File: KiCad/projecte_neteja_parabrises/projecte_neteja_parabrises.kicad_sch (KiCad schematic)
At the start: 0 parts

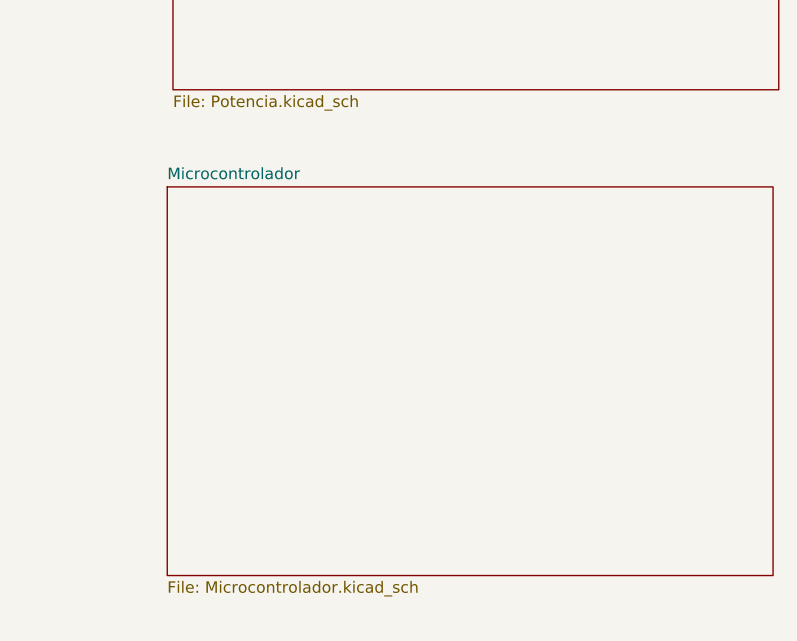
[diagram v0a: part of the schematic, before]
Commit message: huella
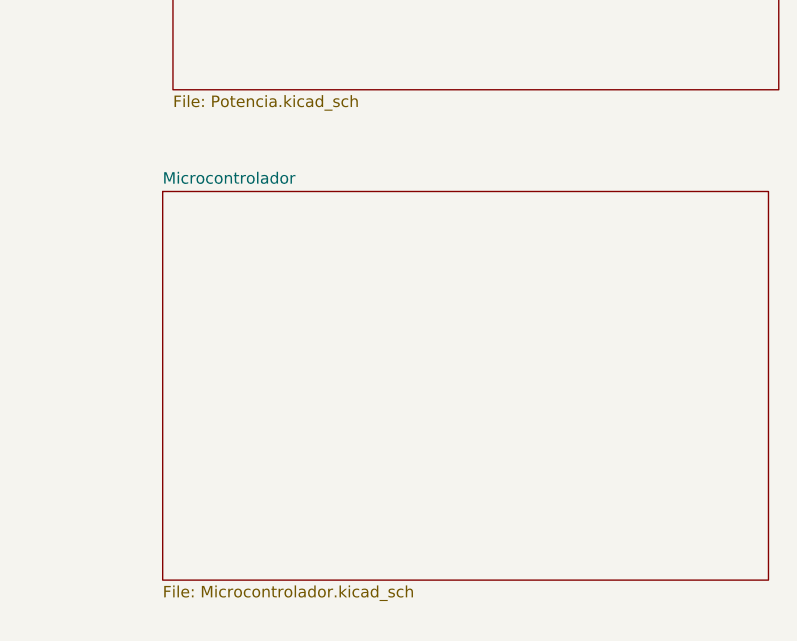
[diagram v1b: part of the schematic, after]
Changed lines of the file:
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@@
 	)
 	(sheet
-		(at 109.855 73.025)
+		(at 109.347 73.533)
 		(size 67.31 43.18)
 		(exclude_from_sim no)
@@
 		)
 		(property "Sheetname" "Microcontrolador"
-			(at 109.855 72.3134 0)
+			(at 109.347 72.8214 0)
 			(effects
 				(font
@@
 		)
 		(property "Sheetfile" "Microcontrolador.kicad_sch"
-			(at 109.855 116.7896 0)
+			(at 109.347 117.2976 0)
 			(effects
 				(font
